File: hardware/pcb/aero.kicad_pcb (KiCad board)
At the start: 4 copper layers, 89 parts, among them CON1 USB-MICRO-B, CON2 MMCX_CONN, J1 CORTEX_DBG_CONN, J2 LiPoly_Conn, Q1 Q_NPN_BEC, SW1 SW_PUSH, U1 STM32L151C8, U2 nRF8001, U3 ms5611, U4 BMX055, U5 AT45DB321E, U6 BQ24040DSQ, U7 TPS783, U8 TPS61041, U9 ZXMHC6A07N8, Y1 Crystal, Y2 Crystal, Y3 32.768KHz, Y4 16MHz

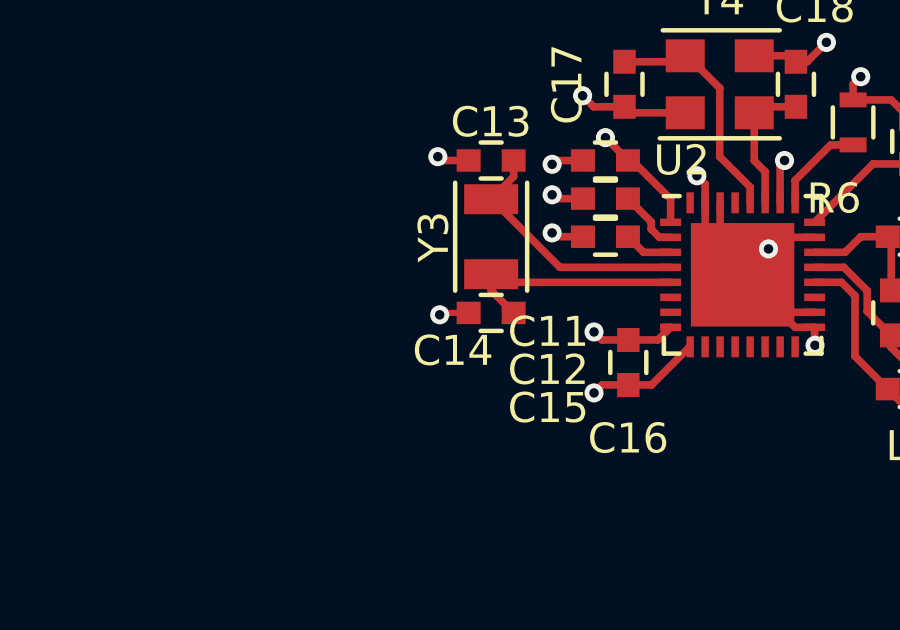
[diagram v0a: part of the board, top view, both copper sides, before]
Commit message: mega commit
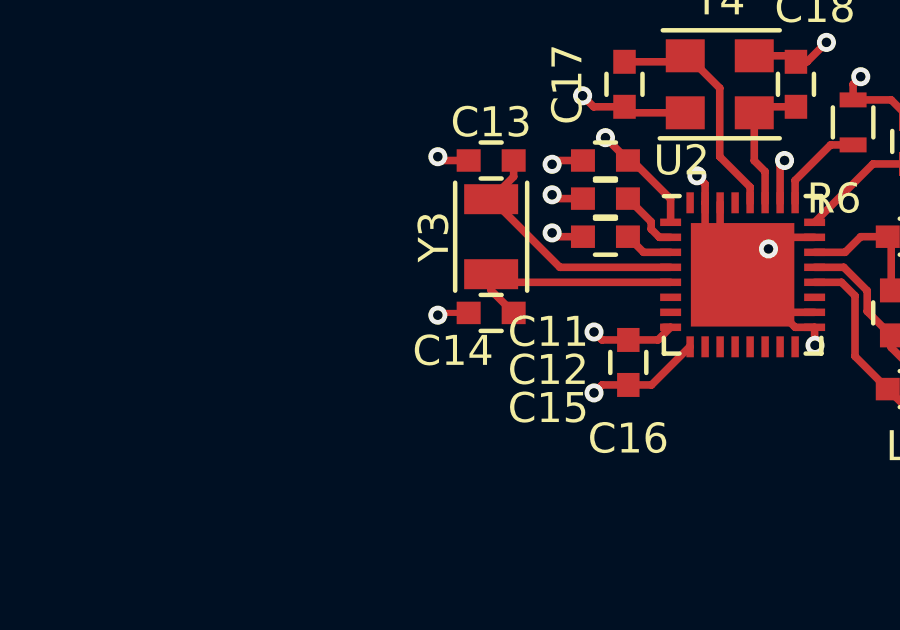
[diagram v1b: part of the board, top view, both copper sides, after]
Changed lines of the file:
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@@
   (segment (start 217.452 99.555) (end 217.437 99.555) (width 0.254) (layer F.Cu) (net 1))
   (segment (start 217.437 99.555) (end 216.166 100.826) (width 0.254) (layer F.Cu) (net 1))
-  (segment (start 210.07 98.425) (end 209.169 98.425) (width 0.2032) (layer F.Cu) (net 2) (status 400000))
-  (via (at 209.1055 98.4885) (size 0.635) (layers F.Cu B.Cu) (net 2))
-  (segment (start 209.169 98.425) (end 209.1055 98.4885) (width 0.2032) (layer F.Cu) (net 2))
+  (segment (start 210.07 98.425) (end 209.1182 98.425) (width 0.2032) (layer F.Cu) (net 2) (status 400000))
+  (via (at 209.042 98.5012) (size 0.635) (layers F.Cu B.Cu) (net 2))
+  (segment (start 209.1182 98.425) (end 209.042 98.5012) (width 0.2032) (layer F.Cu) (net 2))
   (segment (start 189.738 151.626) (end 189.726 151.626) (width 0.2032) (layer F.Cu) (net 2))
   (segment (start 189.726 151.626) (end 188.6585 150.5585) (width 0.2032) (layer F.Cu) (net 2))
@@
   (segment (start 227.9135 102.2985) (end 225.3735 102.2985) (width 0.254) (layer F.Cu) (net 14))
   (segment (start 225.3735 102.2985) (end 224.04 100.965) (width 0.254) (layer F.Cu) (net 14))
-  (segment (start 225.54 95.885) (end 227.85 95.885) (width 0.2032) (layer F.Cu) (net 16) (status C00000))
+  (segment (start 225.54 95.885) (end 227.85 95.885) (width 0.2032) (layer F.Cu) (net 16))
   (segment (start 184.642 156.21) (end 184.642 155.3812) (width 0.508) (layer F.Cu) (net 17))
   (segment (start 184.162 154.9012) (end 184.162 154.178) (width 0.508) (layer F.Cu) (net 17))
